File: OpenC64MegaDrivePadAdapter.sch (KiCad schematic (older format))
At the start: 19 parts, among them J10 DB9_F_TO_C64, J20 DB9_M_TO_PAD, Q1 BC547, Q2 BC547

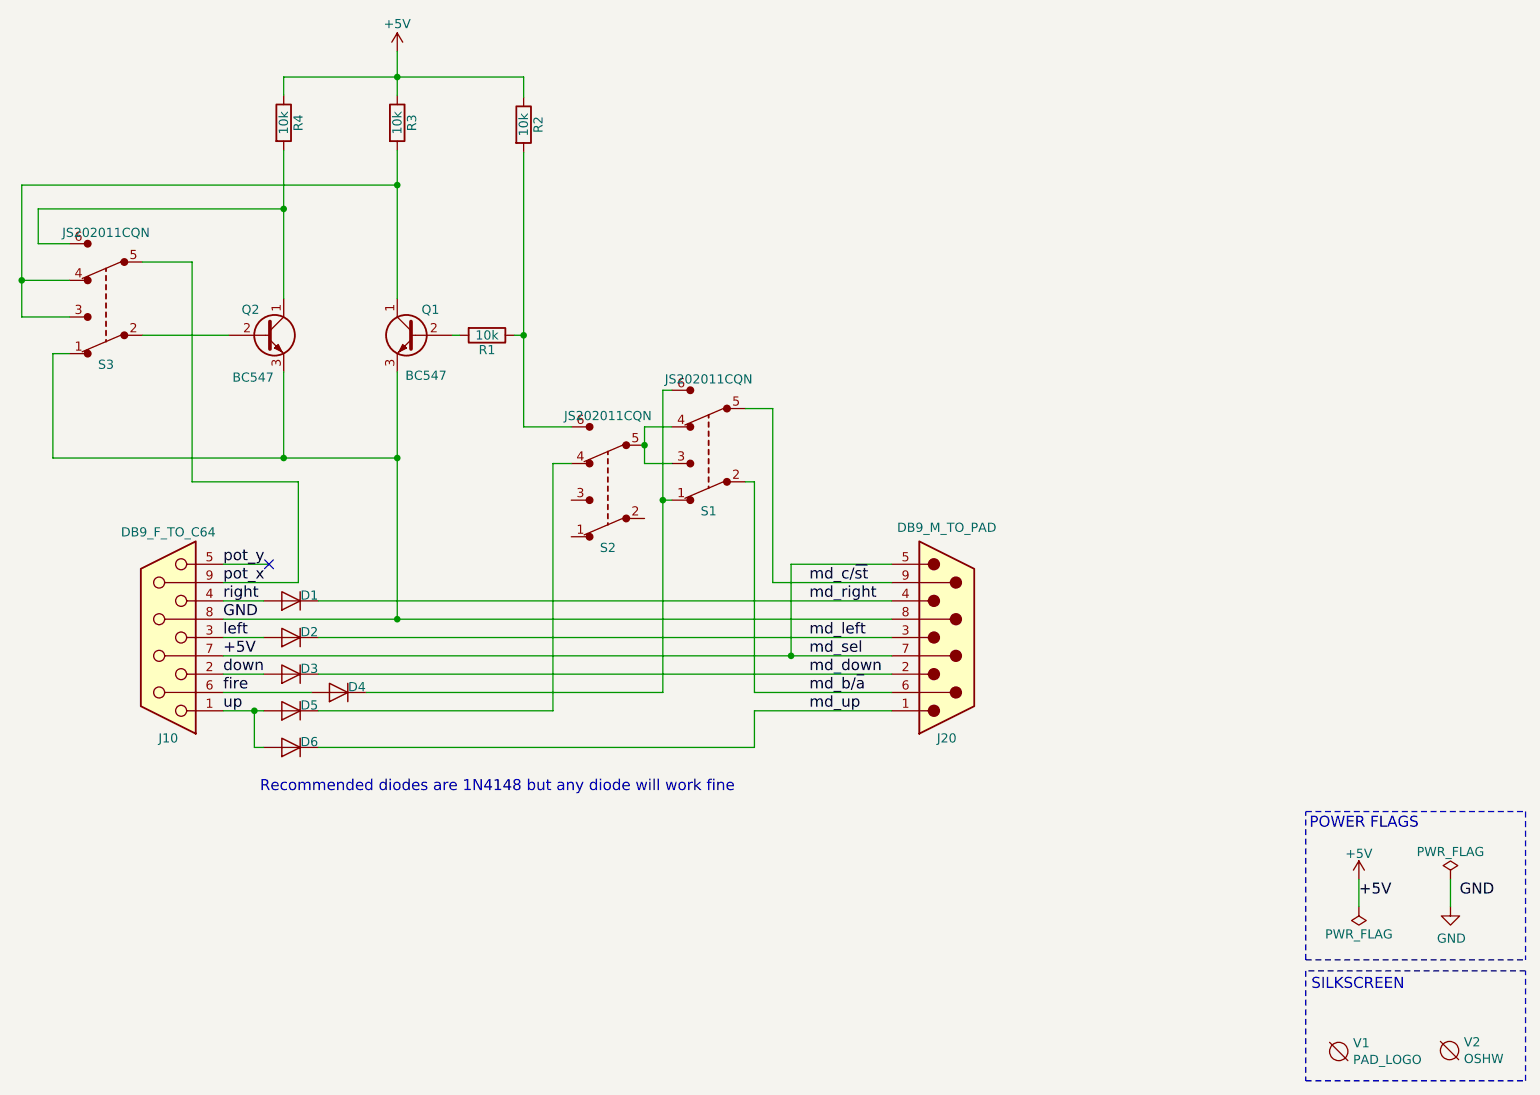
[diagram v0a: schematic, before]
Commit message: rev 6
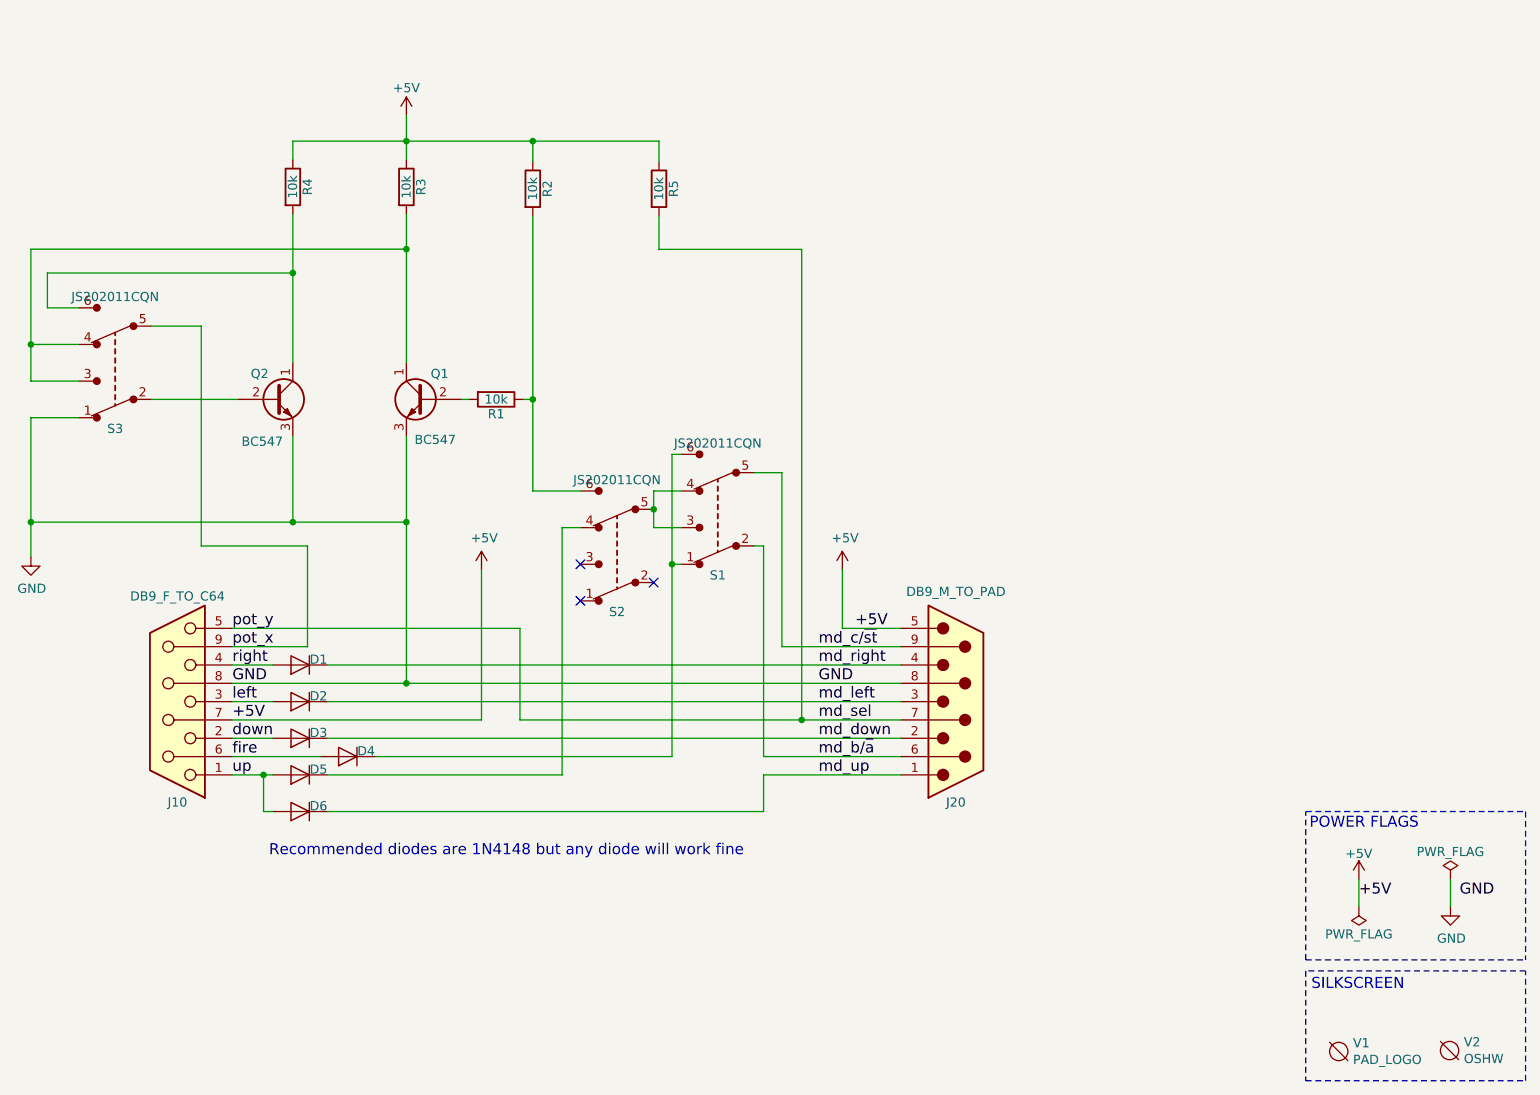
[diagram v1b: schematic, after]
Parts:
- added R5: 10k, Resistor_THT:R_Axial_DIN0204_L3.6mm_D1.6mm_P7.62mm_Horizontal, symbol rescue:R
- D1, D2, D3, D4, D5, D6: footprint Diodes_THT:D_DO-35_SOD27_P7.62mm_Horizontal -> Diode_THT:D_DO-35_SOD27_P7.62mm_Horizontal
- J10: footprint db9:DB_9F -> OpenC64MegaDrivePadAdapter:DB_9F
- J20: footprint w_conn_d-sub:DB_9M -> OpenC64MegaDrivePadAdapter:DB_9M
- Q1, Q2: footprint TO_SOT_Packages_THT:TO-92_Molded_Narrow -> Package_TO_SOT_THT:TO-92L_HandSolder
- R1, R2, R3, R4: footprint Resistors_THT:R_Axial_DIN0204_L3.6mm_D1.6mm_P7.62mm_Horizontal -> Resistor_THT:R_Axial_DIN0204_L3.6mm_D1.6mm_P7.62mm_Horizontal
- S1, S2, S3: footprint Buttons_Switches_THT:SW_CuK_JS202011CQN_DPDT_Straight -> Button_Switch_THT:SW_CuK_JS202011CQN_DPDT_Straight
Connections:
- net +5V: now also R5.1; no longer J20.7
- net pot_y renamed md_sel
- net md_sel: now also J20.7, R5.2
- no-connect marks 1 -> 3
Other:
- moved on the sheet: D1, D2, D3, D4, D5, D6, J10, J20, Q1, Q2, R1, R2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
